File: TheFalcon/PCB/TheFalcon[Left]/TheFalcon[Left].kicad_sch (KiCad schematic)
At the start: 49 parts, among them J1 Conn_01x04_Pin, J2 Conn_02x05_Odd_Even, J3 Conn_01x04_Pin, J5 Conn_01x01, J6 Conn_01x01, SW1 SW_Push, SW2 SW_Push, SW3 SW_DIP_x02, U2 USBLC6-2P6, U3 USBLC6-2P6, U4 AMS1117-3.3, U5 USBLC6-2P6, U6 STM32G431CBTx, Y1 X322516MOB4SI

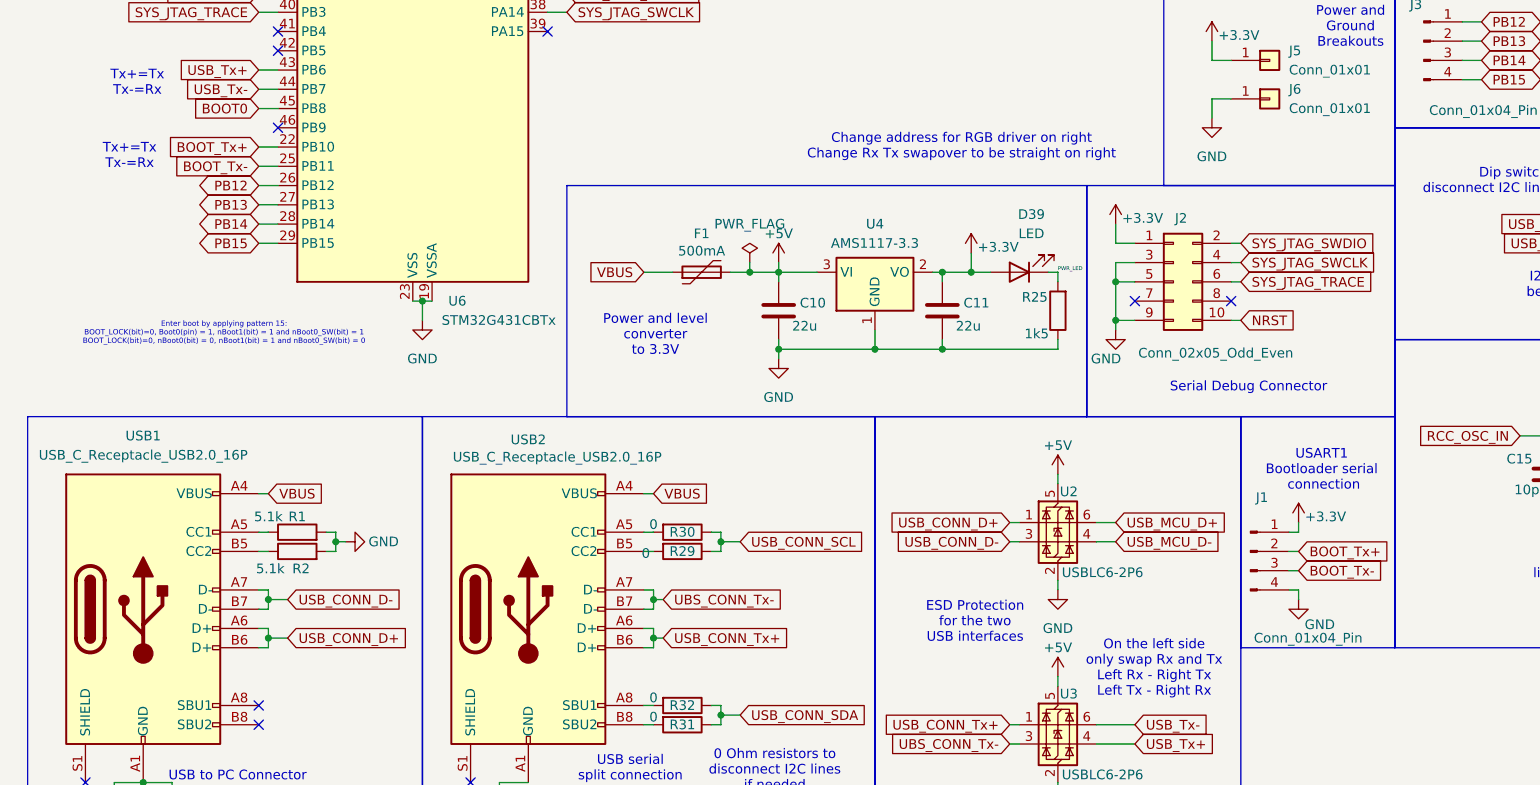
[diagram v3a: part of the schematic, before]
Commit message: Save
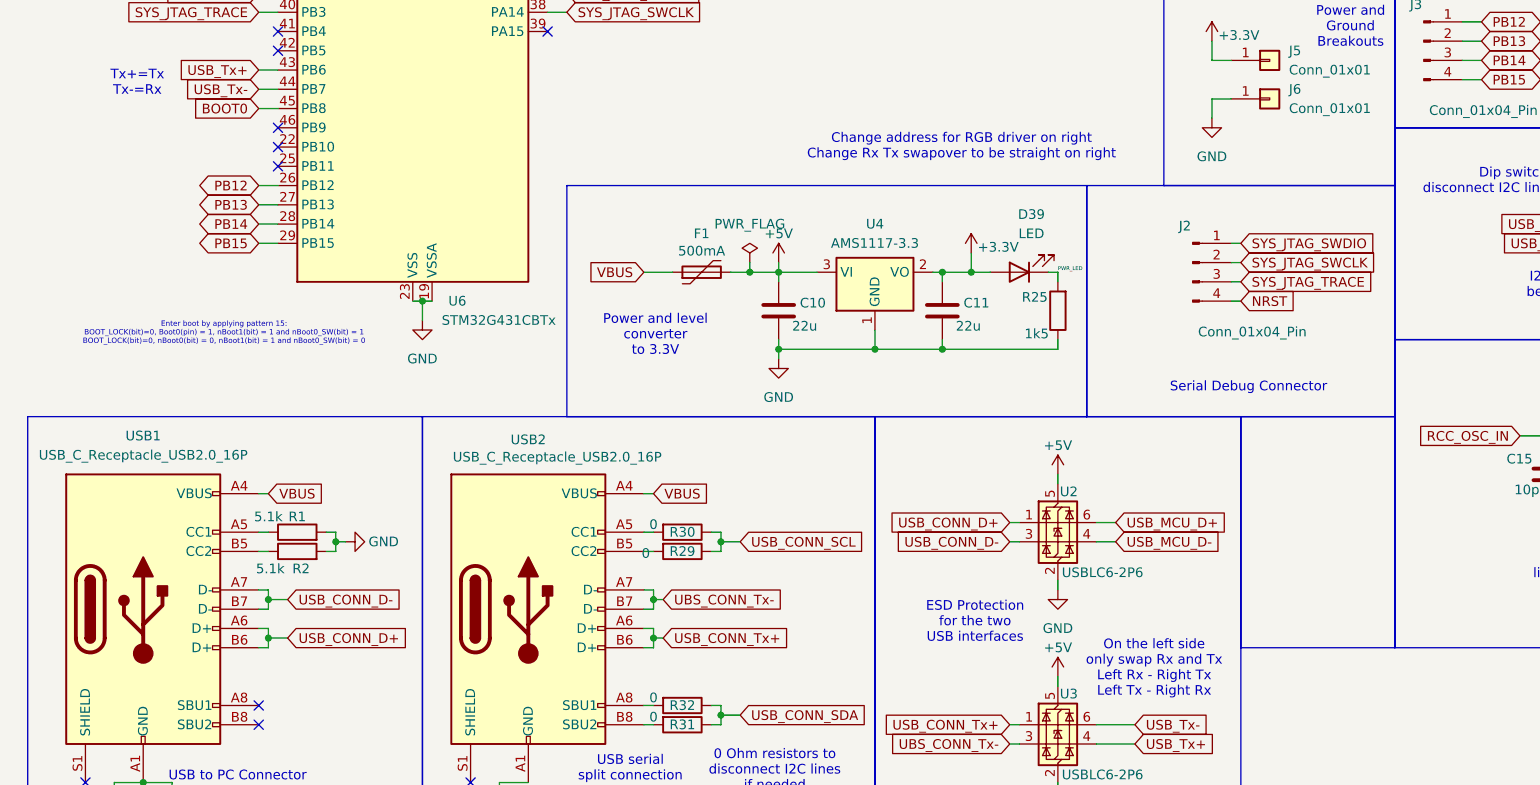
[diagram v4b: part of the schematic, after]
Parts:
- removed J1: Conn_01x04_Pin, Connector_PinSocket_2.54mm:PinSocket_1x04_P2.54mm_Vertical, symbol Connector:Conn_01x04_Pin
- removed J2: Conn_02x05_Odd_Even, Connector_PinSocket_2.54mm:PinSocket_2x05_P2.54mm_Vertical, symbol Connector_Generic:Conn_02x05_Odd_Even
- added J2: Conn_01x04_Pin, Connector_Wire:SolderWire-1sqmm_1x04_P5.4mm_D1.4mm_OD2.7mm, symbol Connector:Conn_01x04_Pin
- C2, C3, C4, C5, C6, C8, C9: footprint Capacitor_SMD:C_0603_1608Metric -> Capacitor_SMD:C_0402_1005Metric
- H1, H2, H3, H4, H5, H6: footprint MountingHole:MountingHole_3.2mm_M3_Pad_Via -> MountingHole:MountingHole_2.2mm_M2_Pad
- J3: footprint Connector_PinSocket_2.54mm:PinSocket_1x04_P2.54mm_Vertical -> Connector_Wire:SolderWire-1sqmm_1x04_P5.4mm_D1.4mm_OD2.7mm
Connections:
- net NRST: now also J2.4 (Pin_4)
- net SYS_JTAG_SWCLK: now also J2.2 (Pin_2)
- net SYS_JTAG_SWDIO: now also J2.1 (Pin_1)
- net SYS_JTAG_TRACE: now also J2.3 (Pin_3)
- net BOOT_Tx+: no longer names the net of U6.22 (PB10)
- net BOOT_Tx-: no longer names the net of U6.25 (PB11)
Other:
- note removed: "USART1 Bootloader serial connection"

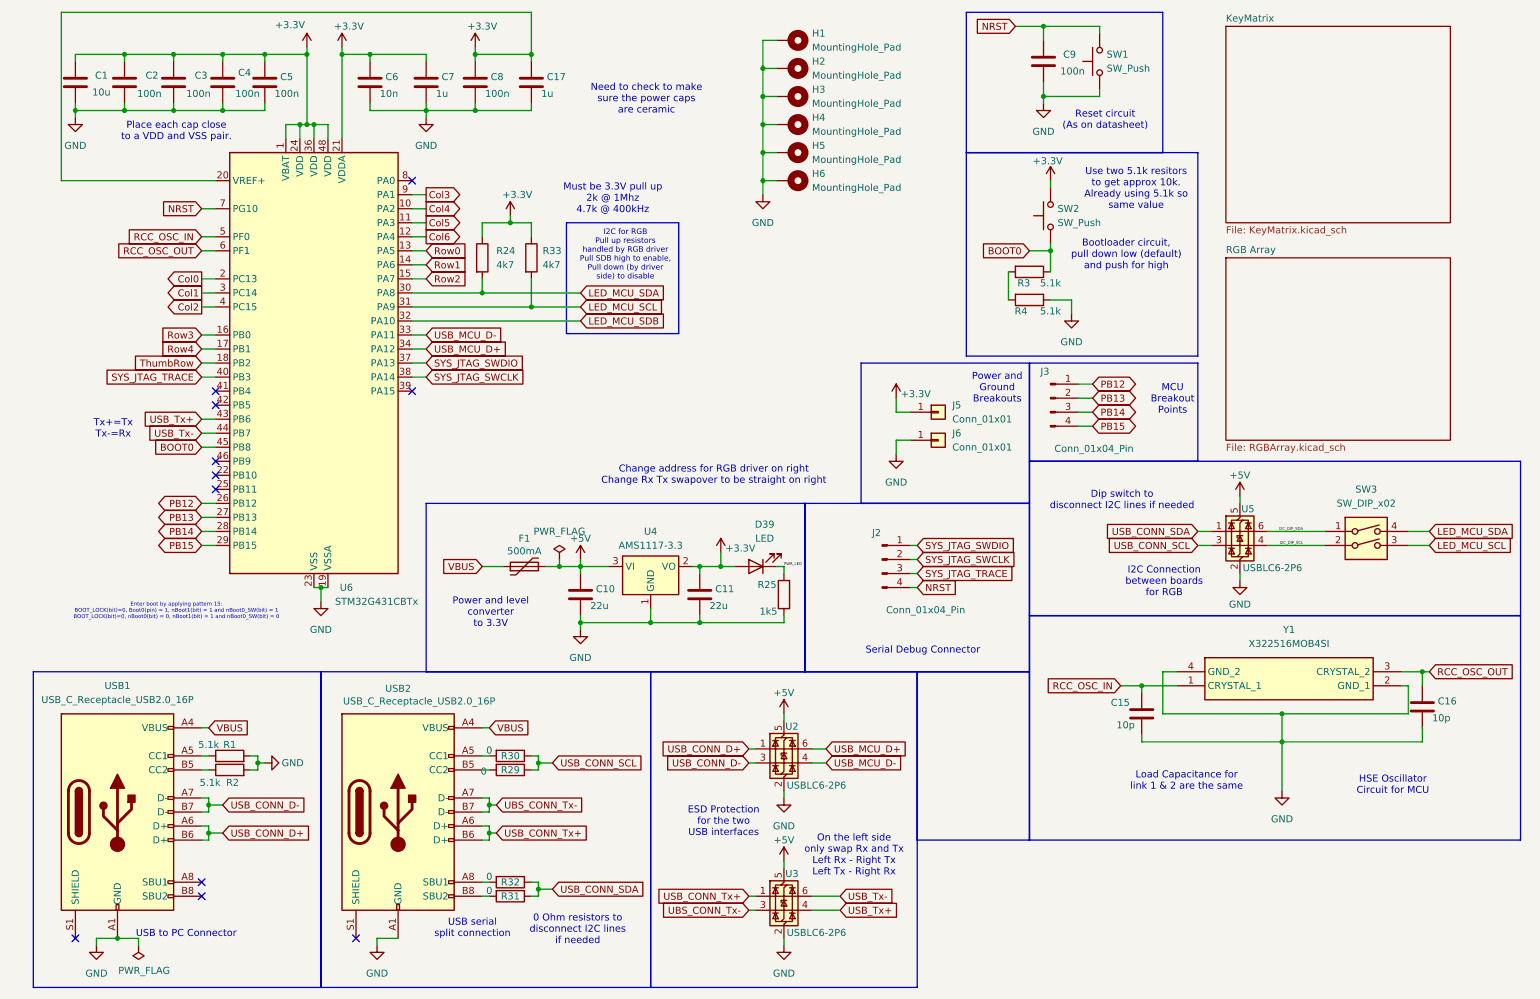
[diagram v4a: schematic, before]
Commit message: Save
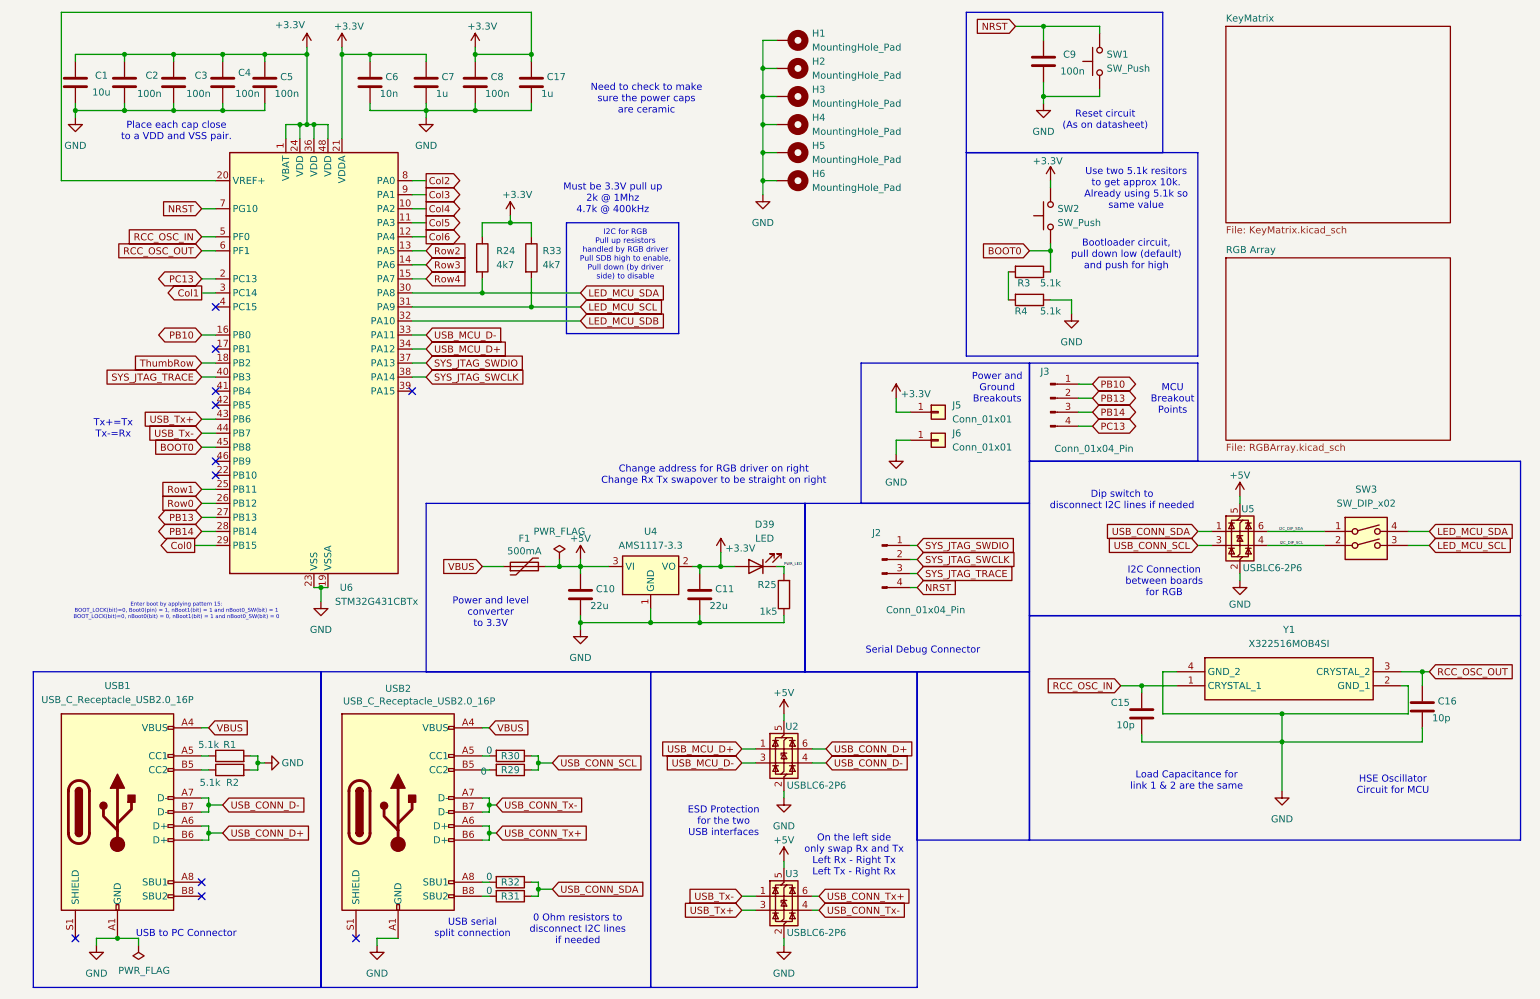
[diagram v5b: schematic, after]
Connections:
- net Col0: now also U6.29 (PB15); no longer U6.2 (PC13)
- net Col2: now also U6.8 (PA0); no longer U6.4 (PC15)
- net Row0: now also U6.26 (PB12); no longer U6.13 (PA5)
- net Row1: now also U6.25 (PB11); no longer U6.14 (PA6)
- net Row2: now also U6.13 (PA5); no longer U6.15 (PA7)
- net Row3: now also U6.14 (PA6); no longer U6.16 (PB0)
- net Row4: now also U6.15 (PA7); no longer U6.17 (PB1)
- net USB_CONN_D+: now also U2.6 (I/O1); no longer U2.1 (I/O1)
- net USB_CONN_D-: now also U2.4 (I/O2); no longer U2.3 (I/O2)
- net USB_CONN_Tx+: now also U3.6 (I/O1); no longer U3.1 (I/O1)
- net USB_MCU_D+: now also U2.1 (I/O1); no longer U2.6 (I/O1)
- net USB_MCU_D-: now also U2.3 (I/O2); no longer U2.4 (I/O2)
- net USB_Tx+: now also U3.3 (I/O2); no longer U3.4 (I/O2)
- net USB_Tx-: now also U3.1 (I/O1); no longer U3.6 (I/O1)
- net PB12 renamed PB10
- net PB10: now also U6.16 (PB0); no longer U6.26 (PB12)
- net PB15 renamed PC13
- net PC13: now also U6.2 (PC13); no longer U6.29 (PB15)
- net UBS_CONN_Tx- renamed USB_CONN_Tx-
- net USB_CONN_Tx-: now also U3.4 (I/O2); no longer U3.3 (I/O2)

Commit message: Saving before I go crazy on PCB
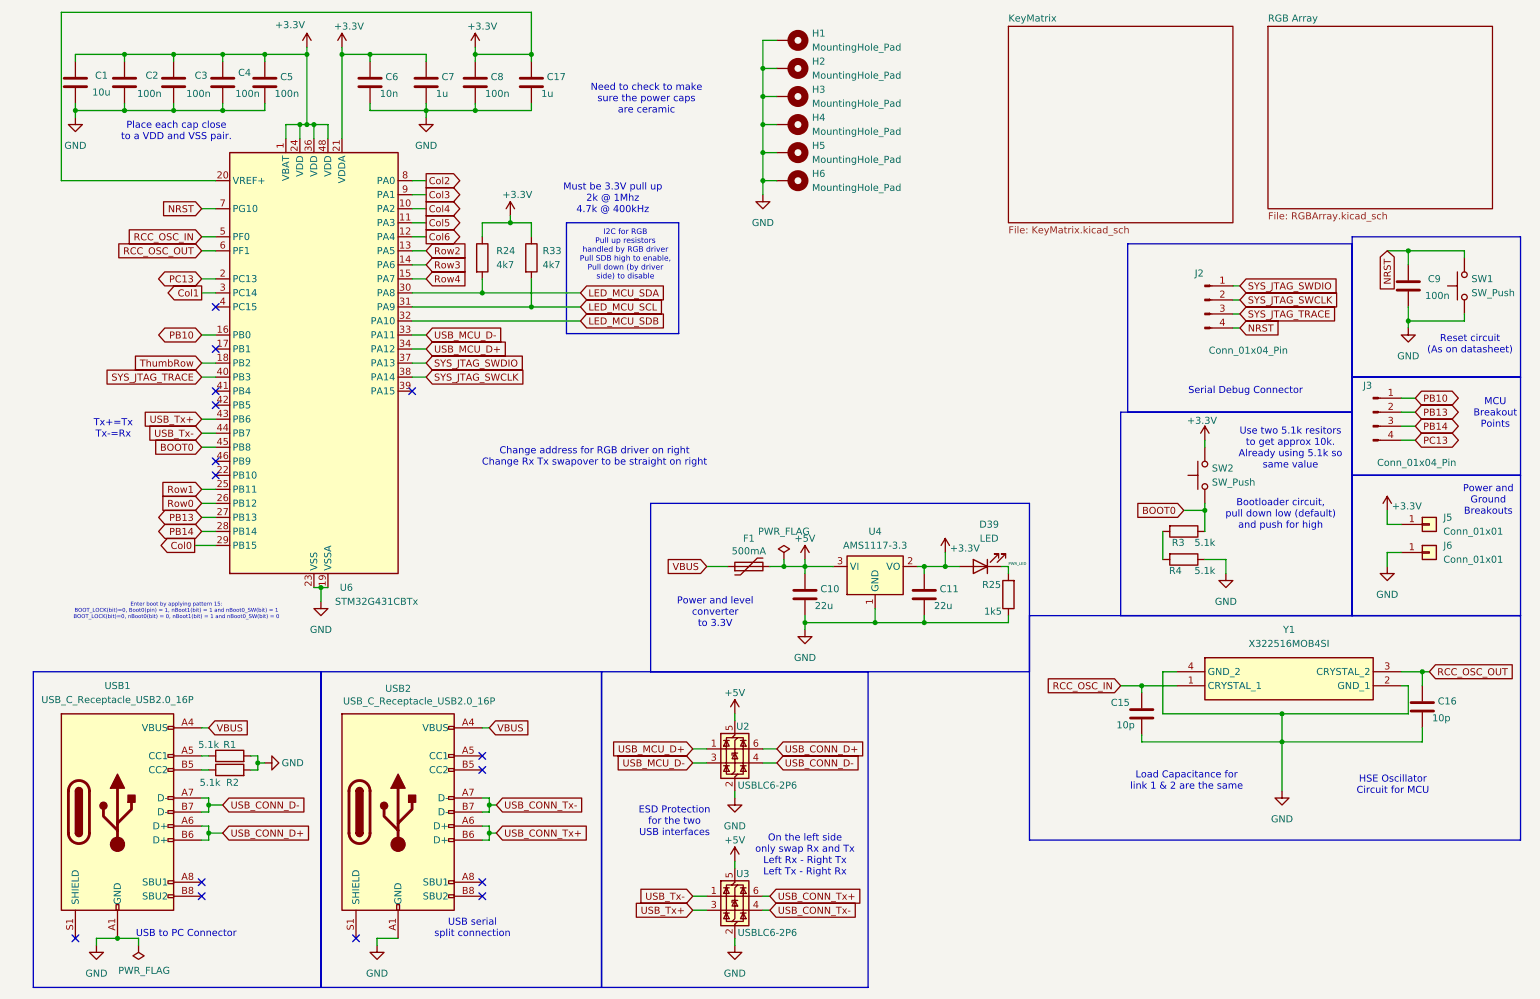
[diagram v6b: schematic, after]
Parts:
- removed R29, R30, R31, R32: 0, Resistor_SMD:R_0805_2012Metric, symbol Device:R
- removed SW3: SW_DIP_x02, Button_Switch_SMD:SW_DIP_SPSTx02_Slide_KingTek_DSHP02TS_W7.62mm_P1.27mm, symbol Switch:SW_DIP_x02
- removed U5: USBLC6-2P6, Package_TO_SOT_SMD:SOT-666, symbol Power_Protection:USBLC6-2P6
- R24, R25, R33: footprint Resistor_SMD:R_0201_0603Metric -> Resistor_SMD:R_0603_1608Metric
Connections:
- no-connect marks 11 -> 15
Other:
- note removed: "0 Ohm resistors to disconnect I2C lines if needed"
- note removed: "Dip switch to disconnect I2C lines if needed"
- note removed: "I2C Connection between boards for RGB"
- moved on the sheet: C10, C11, C9, D39, F1, J2, J3, J5, J6, R25, R3, R4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

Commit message: Save
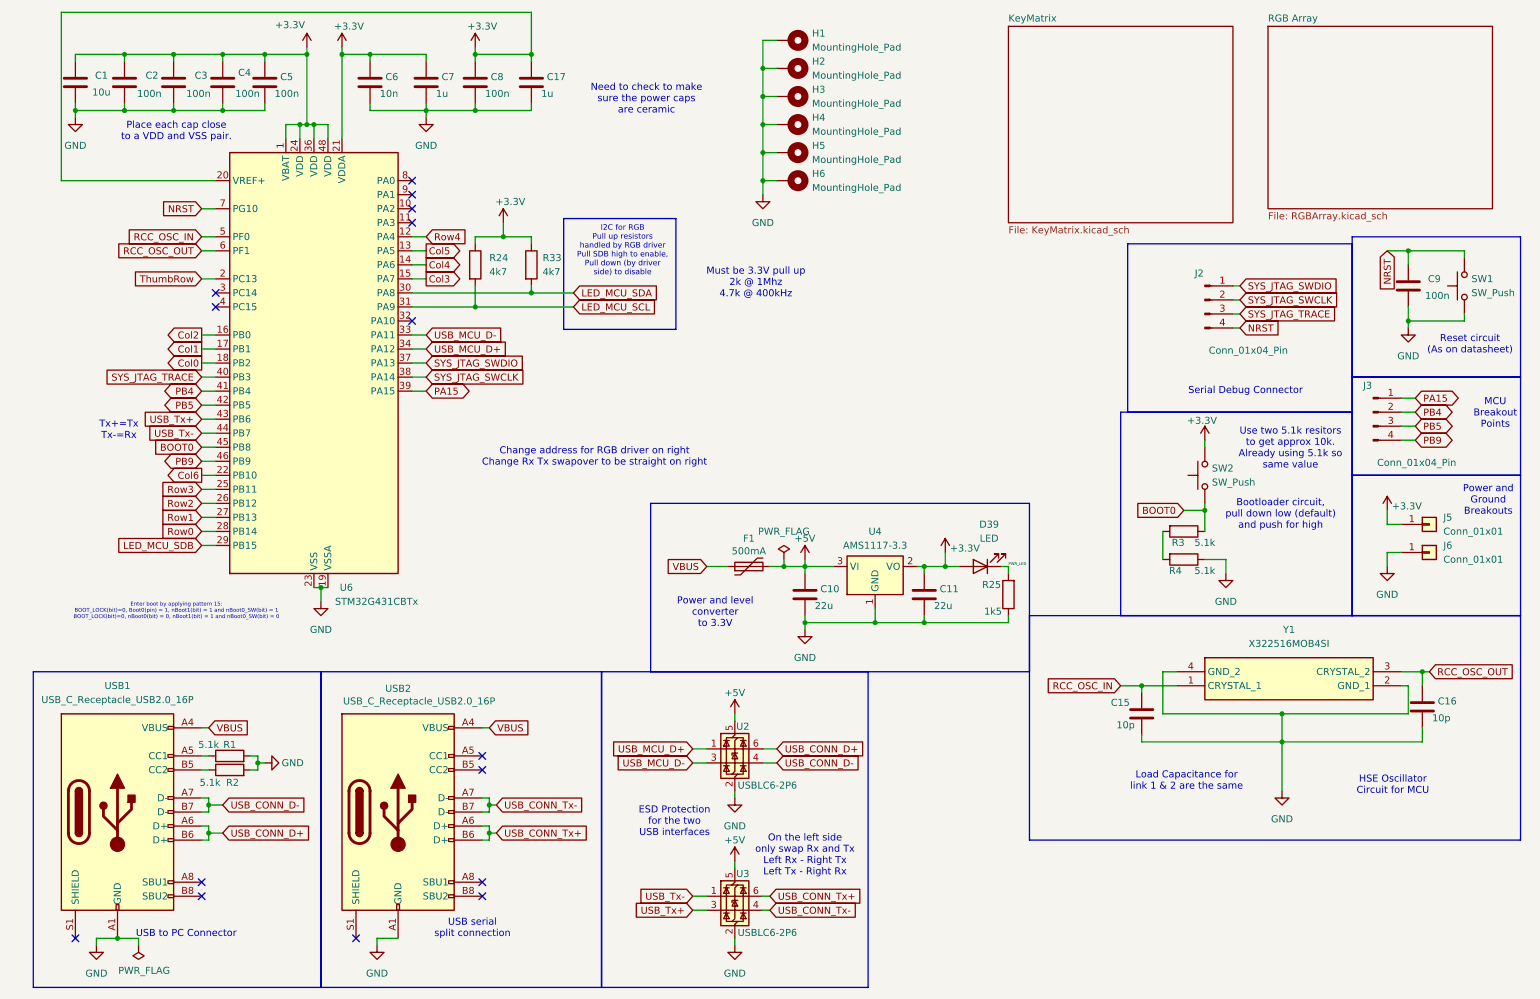
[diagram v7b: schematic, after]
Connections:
- net Col0: now also U6.18 (PB2); no longer U6.29 (PB15)
- net Col1: now also U6.17 (PB1); no longer U6.3 (PC14)
- net Col2: now also U6.16 (PB0); no longer U6.8 (PA0)
- net Col3: now also U6.15 (PA7); no longer U6.9 (PA1)
- net Col4: now also U6.14 (PA6); no longer U6.10 (PA2)
- net Col5: now also U6.13 (PA5); no longer U6.11 (PA3)
- net Col6: now also U6.22 (PB10); no longer U6.12 (PA4)
- net LED_MCU_SCL: now also R24.2; no longer R33.2
- net LED_MCU_SDA: now also R33.2; no longer R24.2
- net LED_MCU_SDB: now also U6.29 (PB15); no longer U6.32 (PA10)
- net Row0: now also U6.28 (PB14); no longer U6.26 (PB12)
- net Row1: now also U6.27 (PB13); no longer U6.25 (PB11)
- net Row2: now also U6.26 (PB12); no longer U6.13 (PA5)
- net Row3: now also U6.25 (PB11); no longer U6.14 (PA6)
- net Row4: now also U6.12 (PA4); no longer U6.15 (PA7)
- net ThumbRow: now also U6.2 (PC13); no longer U6.18 (PB2)
- net PA15: now reaches U6.39 (PA15)
- net PA15: now also J3.1 (Pin_1)
- net PB4: now reaches U6.41 (PB4)
- net PB4: now also J3.2 (Pin_2)
- net PB5: now reaches U6.42 (PB5)
- net PB5: now also J3.3 (Pin_3)
- net PB9: now reaches U6.46 (PB9)
- net PB9: now also J3.4 (Pin_4)
- removed net PB10: J3.1 (Pin_1), U6.16 (PB0)
- removed net PB13: J3.2 (Pin_2), U6.27 (PB13)
- removed net PB14: J3.3 (Pin_3), U6.28 (PB14)
- removed net PC13: J3.4 (Pin_4), U6.2 (PC13)
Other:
- moved on the sheet: R24, R33
